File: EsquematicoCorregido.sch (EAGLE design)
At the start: 45 parts, among them IC1 OPA991TIDCKR, IC10 MCP73831T-2ACI_OT, IC2 AD8226ARZ-RL, IC3 OPA991TIDCKR, IC4 ESP32-S3-WROOM-1-N16R8, IC5 OPA991TIDCKR, IC6 MAX30102EFD+T, IC7 LP38692MP-3.3_NOPB, IC8 LP38692MP-1.8_NOPB, IC9 REF2033AIDDCT, J2 SJ-3523-SMT-TR, J3 USB4216-03-A

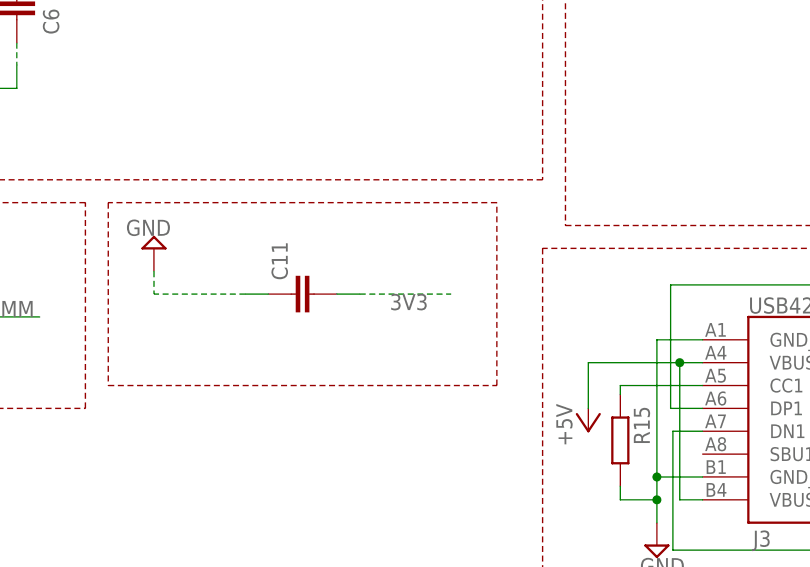
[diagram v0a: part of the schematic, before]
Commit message: ultimo avance
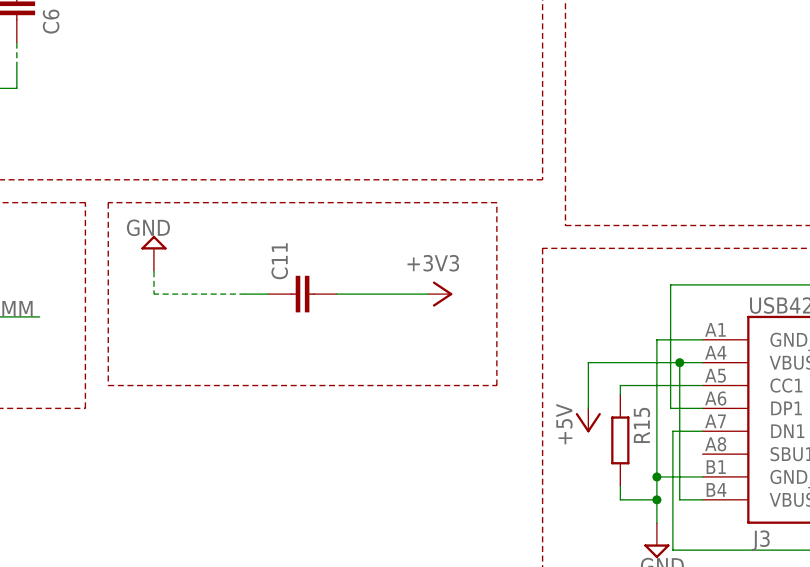
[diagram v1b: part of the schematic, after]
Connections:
- removed net 3V3: C11.2
- net +3V3: now also C11.2
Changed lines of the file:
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@@
 <part name="+3V13" library="supply1" library_urn="urn:adsk.eagle:library:371" deviceset="+3V3" device=""/>
 <part name="P+1" library="supply1" library_urn="urn:adsk.eagle:library:371" deviceset="VCC" device="" value="+1V8"/>
+<part name="+3V14" library="supply1" library_urn="urn:adsk.eagle:library:371" deviceset="+3V3" device=""/>
 </parts>
 <sheets>
@@
 <attribute name="VALUE" x="2.54" y="165.1" size="1.778" layer="96" rot="R90"/>
 </instance>
+<instance part="+3V14" gate="G$1" x="177.8" y="81.28" smashed="yes" rot="R270">
+<attribute name="VALUE" x="172.72" y="83.82" size="1.778" layer="96"/>
+</instance>
 </instances>
 <busses>
@@
 <wire x1="68.58" y1="88.9" x2="68.58" y2="86.36" width="0.1524" layer="91" style="longdash"/>
 </segment>
+<segment>
+<pinref part="C11" gate="G$1" pin="2"/>
+<wire x1="165.1" y1="81.28" x2="175.26" y2="81.28" width="0.1524" layer="91"/>
+<pinref part="+3V14" gate="G$1" pin="+3V3"/>
+</segment>
 </net>
 <net name="N$6" class="0">
@@
 </segment>
 </net>
-<net name="3V3" class="0">
-<segment>
-<wire x1="167.64" y1="81.28" x2="177.8" y2="81.28" width="0.1524" layer="91" style="longdash"/>
-<label x="175.26" y="81.28" size="1.778" layer="95" rot="R180"/>
-<pinref part="C11" gate="G$1" pin="2"/>
-<wire x1="165.1" y1="81.28" x2="167.64" y2="81.28" width="0.1524" layer="91"/>
-</segment>
-</net>
